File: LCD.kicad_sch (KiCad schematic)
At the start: 1 part, among them U3 AP3019AKTR

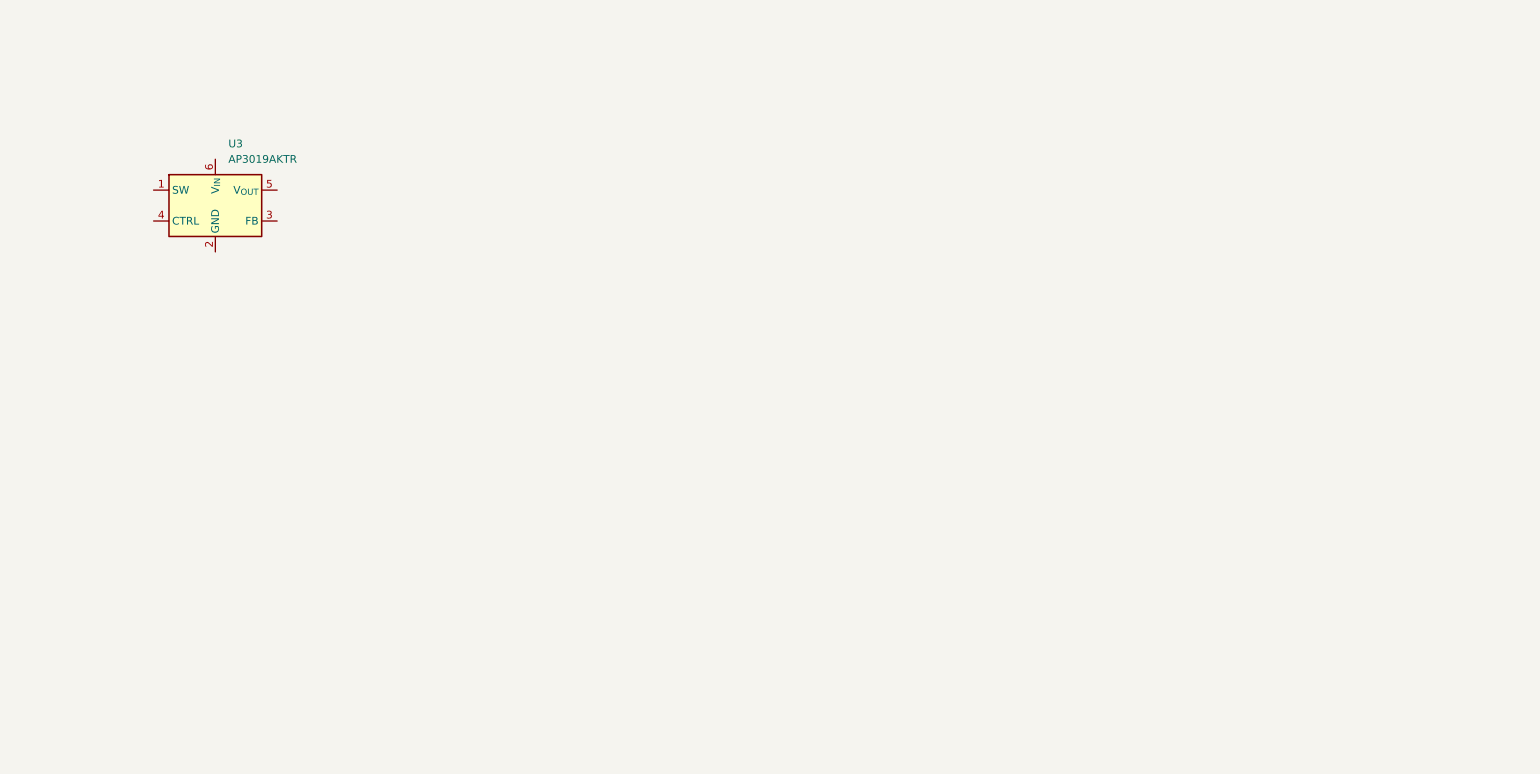
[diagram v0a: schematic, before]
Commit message: LCD connector, backlight, other work
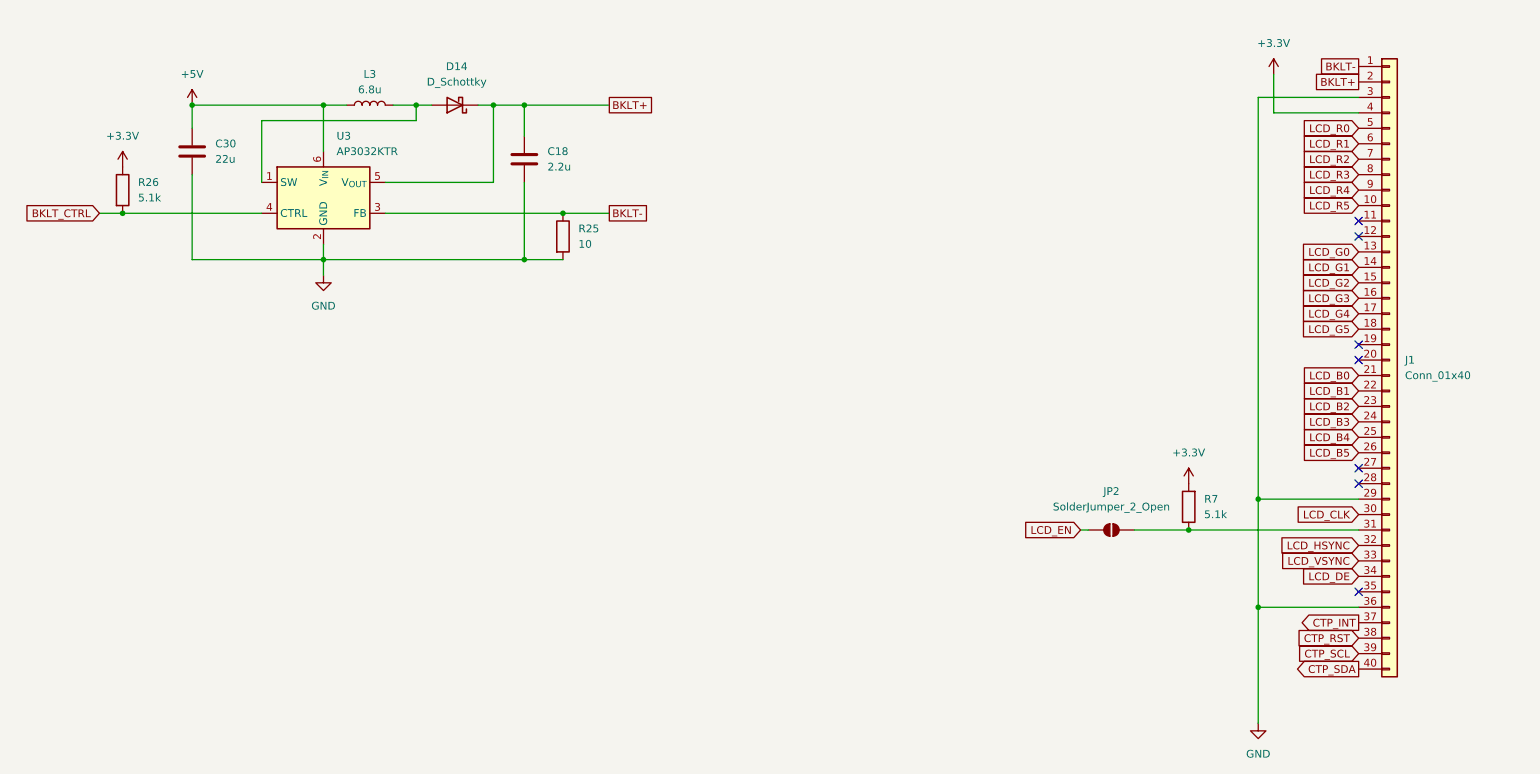
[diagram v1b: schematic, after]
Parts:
- added C18: 2.2u, Capacitor_SMD:C_0603_1608Metric_Pad1.08x0.95mm_HandSolder, symbol Device:C
- added C30: 22u, Capacitor_SMD:C_1206_3216Metric_Pad1.33x1.80mm_HandSolder, symbol Device:C
- added D14: D_Schottky, Diode_SMD:D_SOD-123F, symbol Device:D_Schottky
- added J1: Conn_01x40, Connector_FFC-FPC:TE_3-1734839-9_1x39-1MP_P0.5mm_Horizontal, symbol Connector_Generic:Conn_01x40
- added JP2: SolderJumper_2_Open, Jumper:SolderJumper-2_P1.3mm_Open_RoundedPad1.0x1.5mm, symbol Jumper:SolderJumper_2_Open
- added L3: 6.8u, Inductor_SMD:L_Bourns-SRN4018, symbol Device:L
- added R25: 10, Resistor_SMD:R_0603_1608Metric_Pad0.98x0.95mm_HandSolder, symbol Device:R
- added R26, R7: 5.1k, Resistor_SMD:R_0603_1608Metric_Pad0.98x0.95mm_HandSolder, symbol Device:R
- U3: value AP3019AKTR -> AP3032KTR
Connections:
- net at U3.1 (SW): now also D14.2 (A), L3.2
- net GND: now reaches U3.2 (GND)
- net GND: now also C18.2, C30.2, J1.29 (Pin_29), J1.3 (Pin_3), J1.36 (Pin_36), R25.2
- net BKLT-: now reaches U3.3 (FB)
- net BKLT-: now also J1.1 (Pin_1), R25.1
- net BKLT_CTRL: now reaches U3.4 (CTRL)
- net BKLT_CTRL: now also R26.2
- net BKLT+: now reaches U3.5 (V_{OUT})
- net BKLT+: now also C18.1, D14.1 (K), J1.2 (Pin_2)
- net +5V: now reaches U3.6 (V_{IN})
- net +5V: now also C30.1, L3.1
- new net: J1.31 (Pin_31), JP2.2 (B), R7.1
- new net +3.3V: J1.4 (Pin_4), R26.1, R7.2
- new net CTP_INT: J1.37 (Pin_37)
- new net CTP_RST: J1.38 (Pin_38)
- new net CTP_SCL: J1.39 (Pin_39)
- new net CTP_SDA: J1.40 (Pin_40)
- new net LCD_B0: J1.21 (Pin_21)
- new net LCD_B1: J1.22 (Pin_22)
- new net LCD_B2: J1.23 (Pin_23)
- new net LCD_B3: J1.24 (Pin_24)
- new net LCD_B4: J1.25 (Pin_25)
- new net LCD_B5: J1.26 (Pin_26)
- new net LCD_CLK: J1.30 (Pin_30)
- new net LCD_DE: J1.34 (Pin_34)
- new net LCD_EN: JP2.1 (A)
- new net LCD_G0: J1.13 (Pin_13)
- new net LCD_G1: J1.14 (Pin_14)
- new net LCD_G2: J1.15 (Pin_15)
- new net LCD_G3: J1.16 (Pin_16)
- new net LCD_G4: J1.17 (Pin_17)
- new net LCD_G5: J1.18 (Pin_18)
- new net LCD_HSYNC: J1.32 (Pin_32)
- new net LCD_R0: J1.5 (Pin_5)
- new net LCD_R1: J1.6 (Pin_6)
- new net LCD_R2: J1.7 (Pin_7)
- new net LCD_R3: J1.8 (Pin_8)
- new net LCD_R4: J1.9 (Pin_9)
- new net LCD_R5: J1.10 (Pin_10)
- new net LCD_VSYNC: J1.33 (Pin_33)
- no-connect marks 0 -> 7
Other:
- moved on the sheet: U3

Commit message: preliminary complete schematic
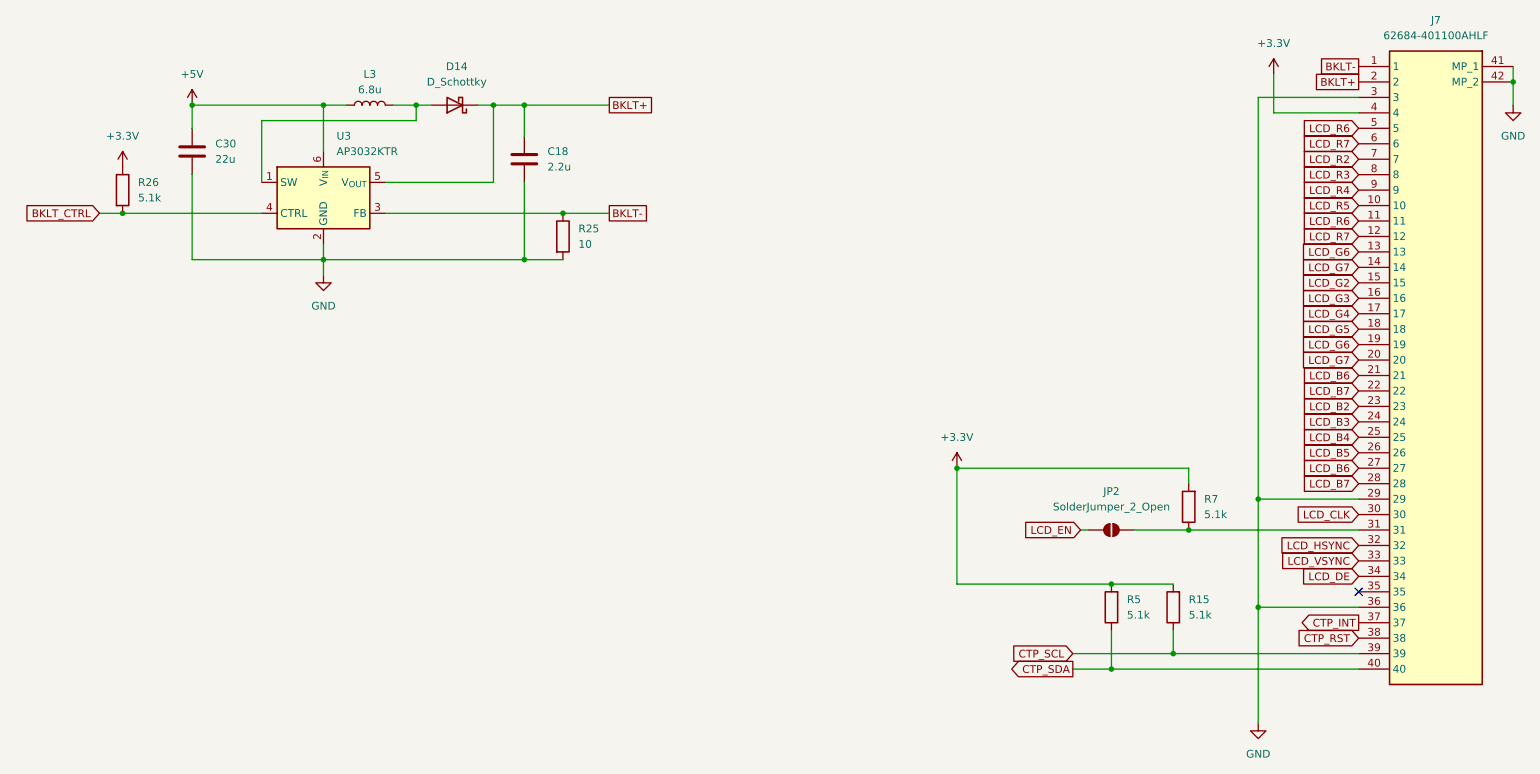
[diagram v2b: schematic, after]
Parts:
- removed J1: Conn_01x40, Connector_FFC-FPC:TE_3-1734839-9_1x39-1MP_P0.5mm_Horizontal, symbol Connector_Generic:Conn_01x40
- added J7: 62684-401100AHLF, 62684401100AHLF, symbol SamacSys_Parts:62684-401100AHLF
- added R15, R5: 5.1k, Resistor_SMD:R_0603_1608Metric_Pad0.98x0.95mm_HandSolder, symbol Device:R
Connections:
- net +3.3V: now also J7.4, R15.2, R5.2
- net BKLT+: now also J7.2
- net BKLT-: now also J7.1
- net CTP_INT: now also J7.37
- net CTP_RST: now also J7.38
- net CTP_SCL: now also J7.39, R15.1
- net CTP_SDA: now also J7.40, R5.1
- net GND: now also J7.29, J7.3, J7.36, J7.41 (MP_1), J7.42 (MP_2)
- net LCD_B2: now also J7.23
- net LCD_B3: now also J7.24
- net LCD_B4: now also J7.25
- net LCD_B5: now also J7.26
- net LCD_CLK: now also J7.30
- net LCD_DE: now also J7.34
- net LCD_G2: now also J7.15
- net LCD_G3: now also J7.16
- net LCD_G4: now also J7.17
- net LCD_G5: now also J7.18
- net LCD_HSYNC: now also J7.32
- net LCD_R2: now also J7.7
- net LCD_R3: now also J7.8
- net LCD_R4: now also J7.9
- net LCD_R5: now also J7.10
- net LCD_VSYNC: now also J7.33
- net at JP2.2 (B), R7.1: now also J7.31
- new net LCD_B6: J7.21, J7.27
- new net LCD_B7: J7.22, J7.28
- new net LCD_G6: J7.13, J7.19
- new net LCD_G7: J7.14, J7.20
- new net LCD_R6: J7.11, J7.5
- new net LCD_R7: J7.12, J7.6
- no-connect marks 7 -> 1
